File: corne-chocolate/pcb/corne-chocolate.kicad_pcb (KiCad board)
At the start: 2 copper layers, 133.8 x 91.4 mm, 98 parts, among them J3 LED, P1 i2c-pin, P2 i2c-pin, SW1 SW_PUSH, SW10 SW_PUSH, SW11 SW_PUSH, SW12 SW_PUSH, SW13 SW_PUSH, SW14 SW_PUSH, SW15 SW_PUSH, SW16 SW_PUSH, SW17 SW_PUSH, SW18 SW_PUSH, SW19 SW_PUSH, SW2 SW_PUSH, SW20 SW_PUSH, SW21 SW_PUSH, SW3 SW_PUSH, SW4 SW_PUSH, SW5 SW_PUSH, SW6 SW_PUSH, SW7 SW_PUSH, SW8 SW_PUSH, SW9 SW_PUSH, U1 ProMicro

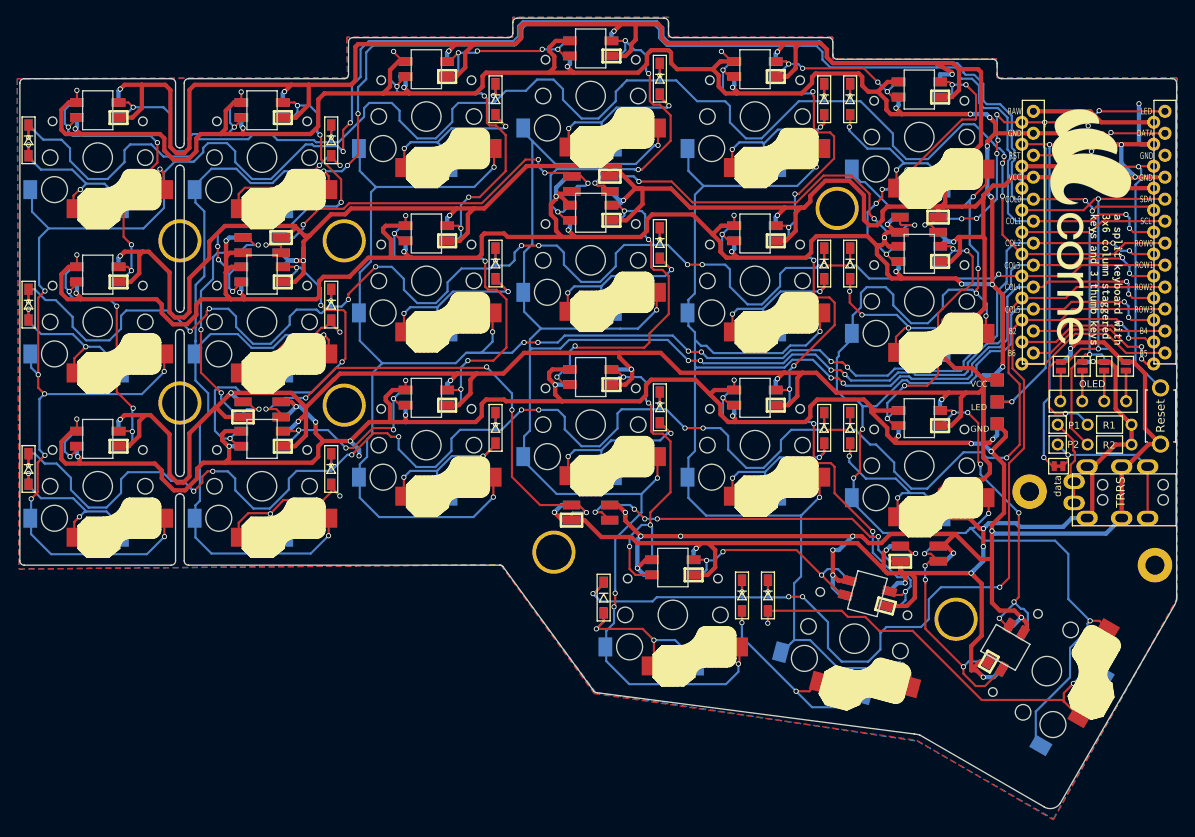
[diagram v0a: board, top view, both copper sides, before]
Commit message: Wireless
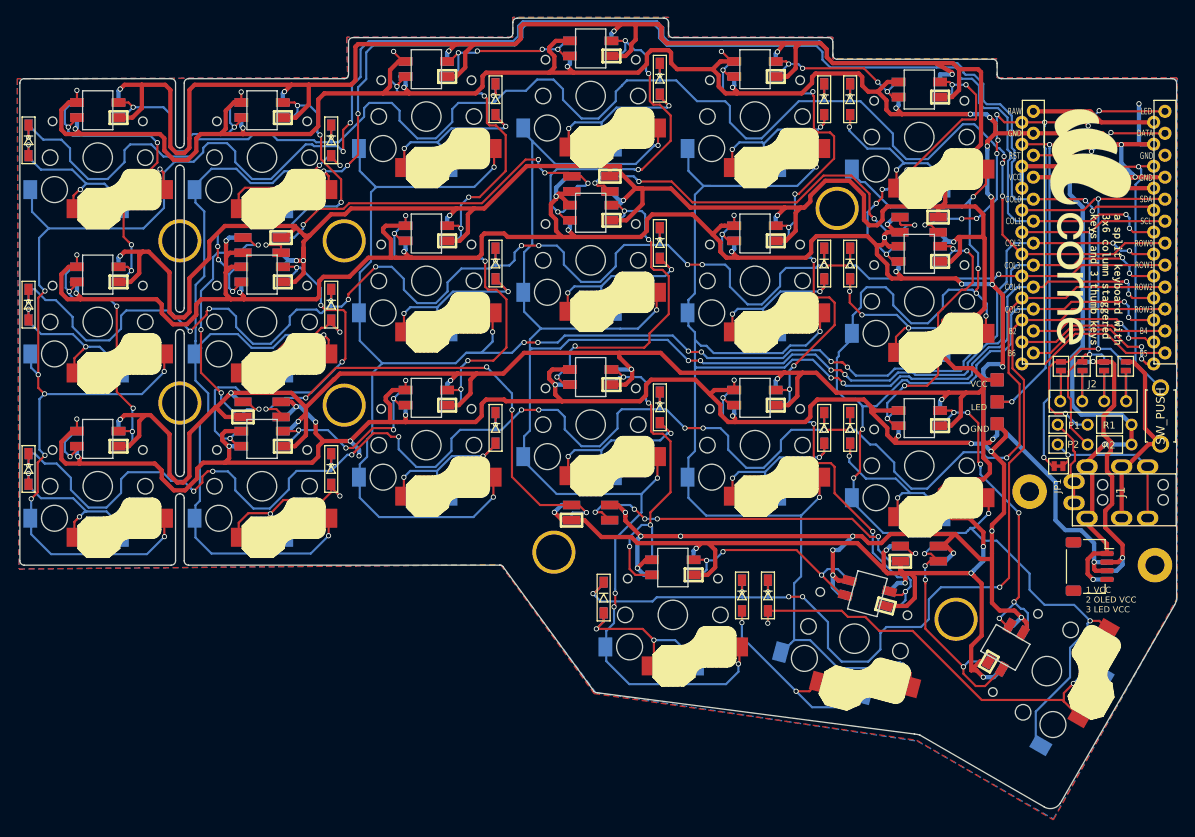
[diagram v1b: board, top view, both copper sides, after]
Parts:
- added J6: Conn_01x04, Allen's Akizukidenshi:JST_SH_SM04B-SRSS-TB_1x04-1MP_P1.00mm_Horizontal-reversible, F.Cu at (184.7, 124.4)
- RSW1: value Reset -> SW_PUSH
- renumbered TRRS to J1, OLED to J2, data to JP1
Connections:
- J3 pad 3: VCC -> VDD
- JP3 pad 1: VCC -> OLED_PWR
- JP8 pad 1: VCC -> OLED_PWR
- L1 pad 4: VCC -> VDD
- L10 pad 4: VCC -> VDD
- L11 pad 4: VCC -> VDD
- L12 pad 4: VCC -> VDD
- L13 pad 1: Net-(L13-Pad1) -> unconnected-(L13-Pad1)
- L13 pad 4: VCC -> VDD
- L14 pad 4: VCC -> VDD
- L15 pad 4: VCC -> VDD
- L16 pad 4: VCC -> VDD
- L17 pad 4: VCC -> VDD
- L18 pad 4: VCC -> VDD
- L19 pad 4: VCC -> VDD
- L2 pad 4: VCC -> VDD
- L20 pad 4: VCC -> VDD
- L21 pad 4: VCC -> VDD
- L3 pad 4: VCC -> VDD
- L4 pad 4: VCC -> VDD
- L5 pad 4: VCC -> VDD
- L6 pad 4: VCC -> VDD
- L7 pad 4: VCC -> VDD
- L8 pad 4: VCC -> VDD
- L9 pad 4: VCC -> VDD
- U1 pad 11: Net-(U1-Pad11) -> unconnected-(U1-Pad11)
- U1 pad 12: Net-(U1-Pad12) -> unconnected-(U1-Pad12)
- U1 pad 13: Net-(U1-Pad13) -> unconnected-(U1-Pad13)
- U1 pad 14: Net-(U1-Pad14) -> unconnected-(U1-Pad14)
- U1 pad 24: Net-(U1-Pad24) -> unconnected-(U1-Pad24)
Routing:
- net VDD: track 0.00 -> 748.7 mm, vias 0 -> 29
- net VCC: track 786.4 -> 76.8 mm, vias 30 -> 3
- net data: track 55.9 -> 0.00 mm, vias 4 -> 0
- net Net-(J1-PadB): track 19.0 -> 74.8 mm, vias 1 -> 5
- net OLED_PWR: track 0.00 -> 33.5 mm, vias 0 -> 2
- net GND: track 816.7 -> 791.8 mm, vias 59 -> 58
- net unconnected-(U1-Pad12): track 0.00 -> 18.9 mm
- net Net-(U1-Pad12): track 18.9 -> 0.00 mm
- net unconnected-(U1-Pad11): track 0.00 -> 17.6 mm
- net Net-(U1-Pad11): track 17.6 -> 0.00 mm
- net Net-(U1-Pad13): track 17.5 -> 0.00 mm, vias 2 -> 0
- net unconnected-(U1-Pad13): track 0.00 -> 17.5 mm, vias 0 -> 2
- net unconnected-(U1-Pad14): track 0.00 -> 16.0 mm, vias 0 -> 2
- net Net-(U1-Pad14): track 16.0 -> 0.00 mm, vias 2 -> 0
- net unconnected-(U1-Pad24): track 0.00 -> 14.4 mm
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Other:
- net class Default removed
- board text added: "1 VCC 2 OLED VCC 3 LED VCC"
- board text added: "3 LED VCC 2 OLED VCC 1 VCC"
- board text added: "Wireless Corne Chocolate v2.1 PCB designed by foostan modified by Allen"
- board text removed: "Corne Chocolate v2.1 PCB designed by foostan"
